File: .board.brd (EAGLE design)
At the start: 25.3 x 23.8 mm, 28 parts, among them U2 FT232RQ, U3 ATTINY1607-MFR, U4 RV-8803, X2 JST_SM02B-SRSS-TB

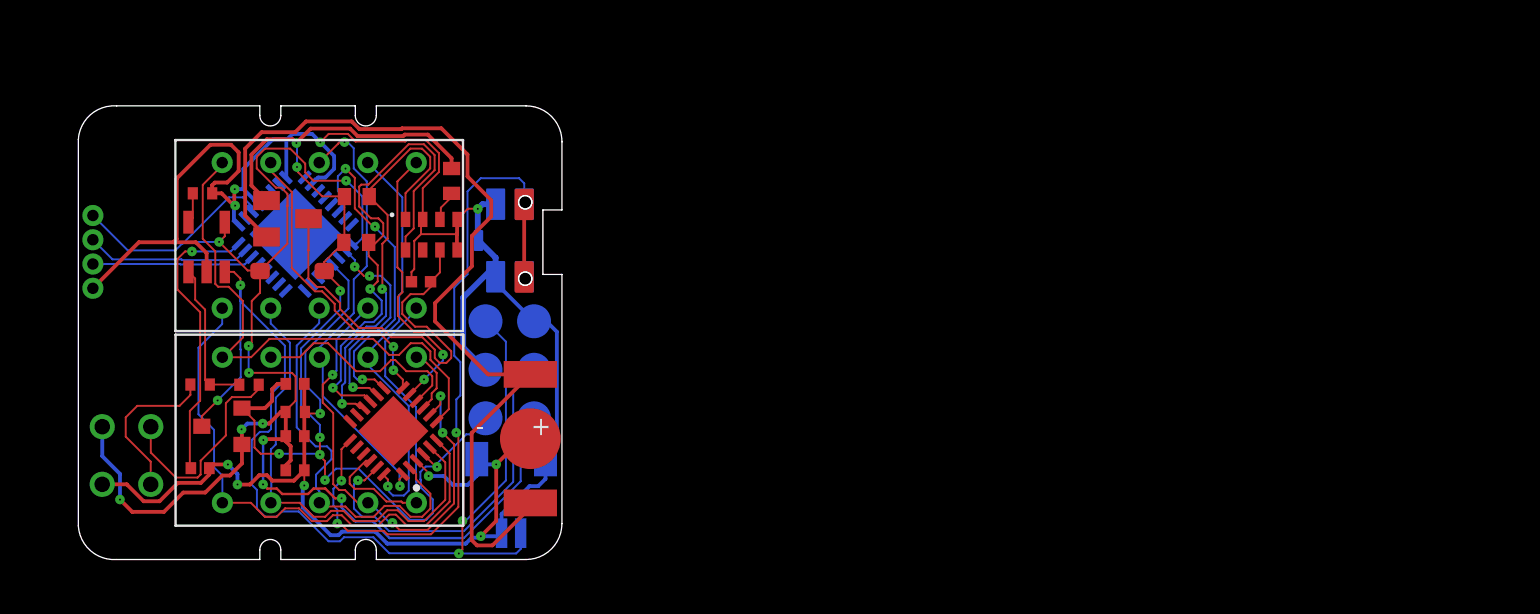
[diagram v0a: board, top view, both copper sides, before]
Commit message: watch file added
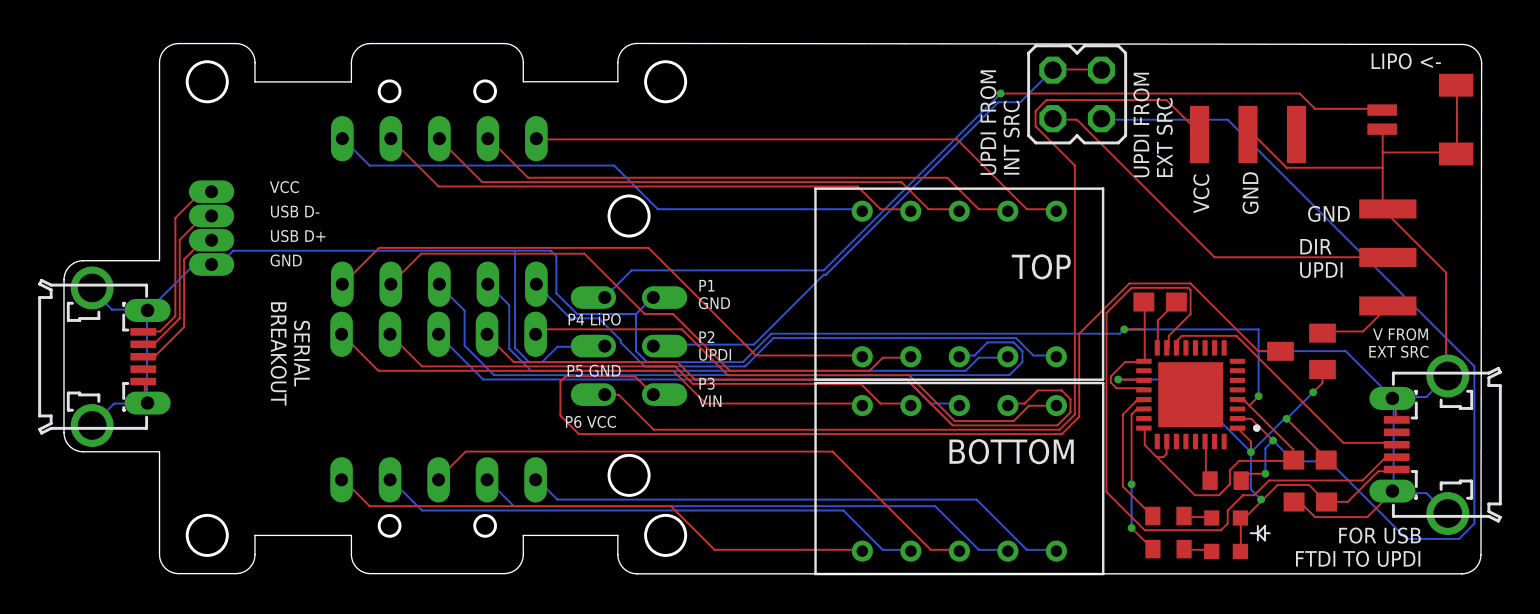
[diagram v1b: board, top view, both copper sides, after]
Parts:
- removed 1.55V-8MAH: BK-414-TR, MY_CLOCK_LIB_COMPONENTS:BK-414-TR
- removed BATTERY_CHARGED_GREEN: GREEN, MY_CLOCK_LIB_COMPONENTS:2MMLED_GREEN
- removed BATT_CONNECTED_YELLOW: ORANGE, MY_CLOCK_LIB_COMPONENTS:2MMLED_YELLOW
- removed BOT: 0.28"-2DIGIT-7SEGEMNT, MY_CLOCK_LIB_COMPONENTS:2_DIGIT_0.28"
- removed C4: 10uF, MY_CAP_LIB:CAPC1005X60
- removed C5: 100nF, MY_CAP_LIB:CAPC1005X60
- removed C6: 10nF, SparkFun-Capacitors:0402-TIGHT
- removed D1: MBR0540, Diodes:SOD-123
- removed R4, R5, R7: 4.7K, ARDUINO_3V_TTL_INTERFACE_2_PI:ADAFRUIT_R0402
- removed R6: 10K, resistor:RESC1005X40
- removed U2: FT232RQ, FT232RQ:QFN50P500X500X90-33N
- removed U3: ATTINY1607-MFR, ATTINY1607-MNR:QFN50P400X400X90-25N
- removed U4: RV-8803, RV-8803:RV-3028
- removed X2: JST_SM02B-SRSS-TB, MY_CLOCK_LIB_COMPONENTS:JST-SM02B-SRSS-TB
- added BOTTOM: 0.28"-2DIGIT-7SEGEMNT, MY_CLOCK_LIB_COMPONENTS:2_DIGIT_0.28"
- added C3: 4.7uF, MY_CLOCK_LIB_COMPONENTS:0603CAP
- added CLOCK_PCB_TEST_PAD_BREAKOUT, DIRECT_UPDI_PROG_PINS: 3PIN_SMT_MALE, keyboard_lib:3PIN__SMT_MALE
- added LIPO_BATT_IN_BREAKOUT: JST_SM02B-SRSS-TB, MY_CLOCK_LIB_COMPONENTS:JST-SM02B-SRSS-TB
- added SERIAL, UPDI: MICROUSB, MY_CLOCK_LIB_COMPONENTS:ZX62D-B-5PA8
- added U$6: 2X0.28_LED_DISP_POGO_PIN_HARNESS, MY_CLOCK_LIB_COMPONENTS:2X0.28_LED_DISP_POGO_PIN_HARNESS
- added U1: FT232RQ, FT232RQ:QFN50P500X500X90-33N
- C1: device MY_CAP_LIB:CAPC1005X60 -> MY_CLOCK_LIB_COMPONENTS:0603CAP
- C2: value 4.7uF -> 100nF; device MY_CAP_LIB:CAPC1005X60 -> MY_CLOCK_LIB_COMPONENTS:0603CAP
- R1, R2: value 470 -> 270/330; device resistor:RESC1005X40 -> MY_0603_RES:RESC1608X60
- R3: value 10K -> 4.7K; device resistor:RESC1005X40 -> MY_0603_RES:RESC1608X60
- U$1: value MCP73831/2_LIPO_CHARGER -> 2X3-P50-E2-POGOPINS; device MY_CLOCK_LIB_COMPONENTS:MCP73831_SOT23-5L -> MY_CLOCK_LIB_COMPONENTS:2X3-P50-E2-POGOPINS
- U$2: value 2X3_PAD_ARRAY -> 1X4-1.27-P50-E2-POGOPINS; device MY_CLOCK_LIB_COMPONENTS:2X3_PAD_ARRAY -> MY_CLOCK_LIB_COMPONENTS:1X4-1.27-P50-E2-POGOPINS
- U$3: value DMG341 -> 0603_LED; device MY_CLOCK_LIB_COMPONENTS:DMG341-P_CHANNEL_MOSFET-SOT23 -> MY_CLOCK_LIB_COMPONENTS:0603_LED
- U$4: value PTS840ESDPMSMTRLF -> 0603_LED; device MY_CLOCK_LIB_COMPONENTS:PTS840ESDPMSMTRLF -> MY_CLOCK_LIB_COMPONENTS:0603_LED
- U$5: value 4X1.27_FEMALE_EMPTY_CONN -> 2X2PIN_JUMPER; device MY_CLOCK_LIB_COMPONENTS:4X1.27_FEMALE_EMPTY_CONN-BACKUP -> MY_CLOCK_LIB_COMPONENTS:2X2PIN_JUMPER
- moved R3 55.6 mm to (60.8, 4.88)
- moved D2 53.5 mm to (64.8, 11.7), turned to 90 degrees
- moved C2 53.1 mm to (65.2, 5.96), turned to 180 degrees
- moved U$3 52.9 mm to (60.8, 1.18)
- moved U$5 52.5 mm to (53.0, 25.1), turned to 180 degrees
- moved R2 51.2 mm to (57.8, 3.03)
- moved R1 48.9 mm to (57.8, 1.29), turned to 0 degrees
- moved C1 46.1 mm to (57.4, 14.2), turned to 180 degrees
- moved U$4 40.2 mm to (60.8, 2.92), flipped to the top, turned to 90 degrees
- moved TOP 33.6 mm to (46.9, 15.2)
- moved U$1 24.0 mm to (30.9, 11.9)
- moved U$2 15.1 mm to (7.72, 18.1), flipped to the top, turned to 0 degrees
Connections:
- removed net !INT: R7.2, U4.6
- removed net COMM1: TOP._9, U3.12
- removed net COMM2: TOP._6, U3.11
- removed net COMM3: BOT._9, U3.10
- removed net COMM4: BOT._6, U3.9
- removed net DOT: BOT._5, TOP._5, U3.22
- removed net N$11: C5.1, U2.16
- removed net N$4: BATT_CONNECTED_YELLOW.K, R1.1
- removed net N$5: R3.1, U$1.5
- removed net N$6: BATTERY_CHARGED_GREEN.A, R2.1
- removed net RX: U2.2, U3.14
- removed net SCL: R4.2, U3.16, U4.8
- removed net SDA: R5.2, U3.15, U4.1
- removed net SEG_A: BOT._7, TOP._7, U3.24
- removed net SEG_B: BOT._8, TOP._8, U3.1
- removed net SEG_C: BOT._3, TOP._3, U3.2
- removed net SEG_D: BOT._2, TOP._2, U3.5
- removed net SEG_E: BOT._1, TOP._1, U3.6
- removed net SEG_F: BOT._10, TOP._10, U3.7
- removed net SEG_G: BOT._4, TOP._4, U3.8
- removed net SW1: U$4.3, U$4.4, U$4.B3, U$4.B4, U3.19
- removed net TX: U2.30, U3.13
- removed net USBDM: U$5.P$2, U2.15
- removed net USBDP: U$5.P$3, U2.14
- removed net VBATT: 1.55V-8MAH.1+, 1.55V-8MAH.2+, D2.2
- removed net VDD1: C6.1, D2.3, U4.3
- new net 3V3OUT: C1.1, U1.16
- new net B1: BOTTOM._1, U$6.BOT1
- new net B10: BOTTOM._10, U$6.BOT10
- new net B2: BOTTOM._2, U$6.BOT2
- new net B3: BOTTOM._3, U$6.BOT3
- new net B4: BOTTOM._4, U$6.BOT4
- new net B5: BOTTOM._5, U$6.BOT5
- new net B6: BOTTOM._6, U$6.BOT6
- new net B7: BOTTOM._7, U$6.BOT7
- new net B8: BOTTOM._8, U$6.BOT8
- new net B9: BOTTOM._9, U$6.BOT9
- new net CBUS0: R1.1, U1.22
- new net CBUS1: R2.1, U1.21
- new net N$1: R1.2, U$3.C
- new net SER_USB_DM: SERIAL.2, U$2.P$2
- new net SER_USB_DP: SERIAL.3, U$2.P$3
- new net SER_VCC: SERIAL.1, U$2.P$1
- new net T1: TOP._1, U$6.TOP1
- new net T10: TOP._10, U$6.TOP10
- new net T2: TOP._2, U$6.TOP2
- new net T3: TOP._3, U$6.TOP3
- new net T4: TOP._4, U$6.TOP4
- new net T5: TOP._5, U$6.TOP5
- new net T6: TOP._6, U$6.TOP6
- new net T7: TOP._7, U$6.TOP7
- new net T8: TOP._8, U$6.TOP8
- new net T9: TOP._9, U$6.TOP9
- new net TXD: R3.1, U1.30
- new net UPDI_DIR: DIRECT_UPDI_PROG_PINS.2, U$5.4
- new net UPDI_PROG_DM: U1.15, UPDI.2
- new net UPDI_PROG_DP: U1.14, UPDI.3
- new net UPDI_TRANS: R3.2, U$5.2, U1.2
- new net VIN: D2.3, U$1.6
- new net V_DIR: D2.2, DIRECT_UPDI_PROG_PINS.1
- net EXP: now also U1.33; no longer U2.33
- net GND: now also C3.2, CLOCK_PCB_TEST_PAD_BREAKOUT.2, DIRECT_UPDI_PROG_PINS.3, LIPO_BATT_IN_BREAKOUT.1, LIPO_BATT_IN_BREAKOUT.M1, LIPO_BATT_IN_BREAKOUT.M2, SERIAL.5, SERIAL.S1, SERIAL.S2, SERIAL.S3, SERIAL.S4, U$1.4, U$2.P$4, U1.17, U1.20, U1.24, U1.26, U1.4, UPDI.5, UPDI.S1, UPDI.S2, UPDI.S3, UPDI.S4; no longer 1.55V-8MAH.-, BATTERY_CHARGED_GREEN.K, C4.2, C5.2, C6.2, R3.2, R6.1, U$2.2, U$2.6, U$4.1, U$4.2, U$4.5, U$5.P$4, U2.17, U2.20, U2.24, U2.26, U2.4, U3.3, U4.4, U4.5, U4.7, X2.1, X2.M1, X2.M2
- net N$2: now also U$4.C; no longer R1.2, U$1.1
- net UPDI: now also U$1.5, U$5.1, U$5.3; no longer U$2.5, U3.23
- net VCC: now also CLOCK_PCB_TEST_PAD_BREAKOUT.3, U$1.3; no longer C4.1, D1.C, D2.1, R4.1, R5.1, R7.1, U$2.3, U$3.2, U3.4
- net V_LIPO: now also LIPO_BATT_IN_BREAKOUT.2, U$1.1; no longer U$1.3, U$2.1, U$3.3, X2.2
- net V_USB: now also C3.1, D2.1, U$3.A, U$4.A, U1.1, U1.19, UPDI.1; no longer BATT_CONNECTED_YELLOW.A, C1.1, D1.A, R6.2, U$1.4, U$2.4, U$3.1, U$5.P$1, U2.1, U2.19
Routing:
- net VIN: track 0.00 -> 52.5 mm
- net V_USB: track 87.1 -> 35.0 mm, vias 10 -> 5
- net UPDI_TRANS: track 0.00 -> 51.8 mm, vias 0 -> 2
- net VBATT: track 48.9 -> 0.00 mm
- net SW1: track 41.1 -> 0.00 mm, vias 3 -> 0
- net GND: track 136.6 -> 176.1 mm, vias 11 -> 2
- net T3: track 0.00 -> 38.3 mm
- net B7: track 0.00 -> 37.3 mm
- net UPDI_PROG_DM: track 0.00 -> 35.9 mm
- net T4: track 0.00 -> 30.7 mm
- net T2: track 0.00 -> 30.7 mm
- net T1: track 0.00 -> 30.4 mm
- net T5: track 0.00 -> 30.1 mm
- net B3: track 0.00 -> 30.1 mm
- net B6: track 0.00 -> 29.7 mm
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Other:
- board size 25.3 x 23.8 mm -> 74.2 x 27.8 mm
- board text added: "DIR UPDI"
- board text added: "FOR USB FTDI TO UPDI"
- board text added: "GND"
- board text added: "LIPO <-"
- board text added: "P1 GND"
- board text added: "P2 UPDI"
- board text added: "P3 VIN"
- board text added: "P4 LiPO"
- board text added: "P5 GND"
- board text added: "P6 VCC"
- board text added: "SERIAL BREAKOUT"
- board text added: "UPDI FROM EXT SRC"
- board text added: "UPDI FROM INT SRC"
- board text added: "V FROM EXT SRC"
- board text added: "VCC"
- board text added: "VCC USB D- USB D+ GND"
- board text removed: "+"
- board text removed: "-"
- board text removed: "P1"
- board text removed: "P2"
- board text removed: "P3"
- board text removed: "P4"
- board text removed: "P5"
- board text removed: "P6"
